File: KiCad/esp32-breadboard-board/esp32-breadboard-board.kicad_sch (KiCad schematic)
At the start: 23 parts, among them J1 USB_C_Receptacle_USB2.0_14P, J2 Conn_01x22_Pin, J3 Conn_01x22_Pin, SW1 BOOT, SW2 EN, U1 ESP32-S3-WROOM-1, U2 USBLC6-2SC6, U3 SGM2212-3.3XKC3G

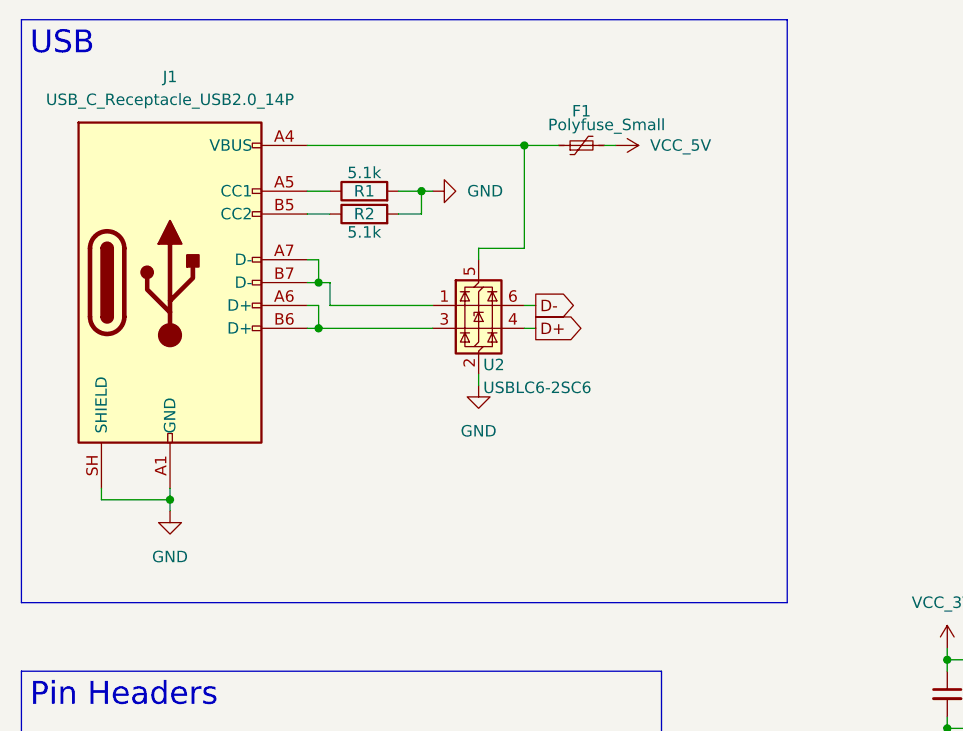
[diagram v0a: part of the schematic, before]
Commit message: Journal P2
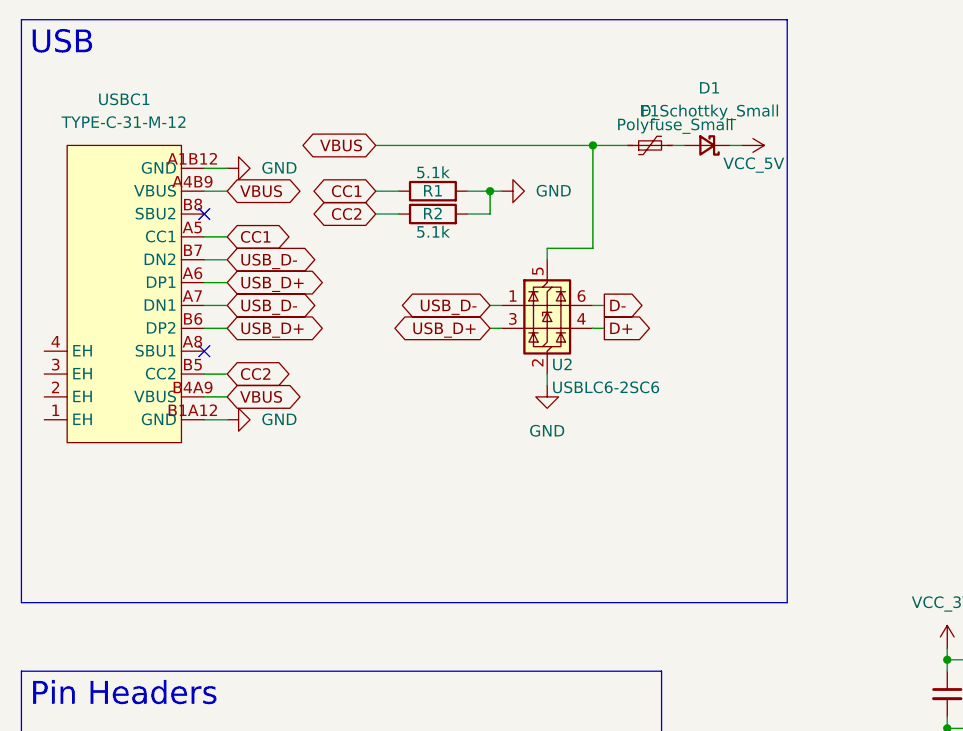
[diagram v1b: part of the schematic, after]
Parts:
- removed J1: USB_C_Receptacle_USB2.0_14P, symbol Connector:USB_C_Receptacle_USB2.0_14P
- added D1: D_Schottky_Small, easyeda2kicad:SOD-123_L2.7-W1.6-LS3.7-RD, symbol Device:D_Schottky_Small
- added USBC1: TYPE-C-31-M-12, easyeda2kicad:USB-C_SMD-TYPE-C-31-M-12_1, symbol easyeda2kicad:TYPE-C-31-M-12
- C10, C11, C7: footprint (none) -> Capacitor_SMD:C_0603_1608Metric
- C12, C14, C8, C9: footprint (none) -> Capacitor_SMD:C_0402_1005Metric
- D5: footprint (none) -> LED_SMD:LED_0603_1608Metric
- F1: footprint (none) -> Fuse:Fuse_0402_1005Metric
- J2, J3: footprint (none) -> Connector_PinHeader_2.54mm:PinHeader_1x20_P2.54mm_Vertical
- R1, R2, R3, R4, R5, R6: footprint (none) -> Resistor_SMD:R_0402_1005Metric
- SW1, SW2: footprint (none) -> easyeda2kicad:SW-SMD_L3.9-W3.0-P4.45
- U1: footprint RF_Module:ESP32-S3-WROOM-1 -> easyeda2kicad:WIFIM-SMD_ESP32-S3-WROOM-1-N8
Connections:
- net GND: now also USBC1.A1B12 (GND), USBC1.B1A12 (GND)
- net VCC_5V: now also D1.1 (K); no longer F1.2
- net VBUS: now reaches F1.1, U2.5 (VBUS)
- net VBUS: now also USBC1.A4B9 (VBUS), USBC1.B4A9 (VBUS)
- net CC1: now reaches R1.1
- net CC1: now also USBC1.A5 (CC1)
- net USB_D+: now reaches U2.3 (I/O2)
- net USB_D+: now also USBC1.A6 (DP1), USBC1.B6 (DP2)
- net USB_D-: now reaches U2.1 (I/O1)
- net USB_D-: now also USBC1.A7 (DN1), USBC1.B7 (DN2)
- net CC2: now reaches R2.1
- net CC2: now also USBC1.B5 (CC2)
- new net: D1.2 (A), F1.2
- no-connect marks 0 -> 2
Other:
- moved on the sheet: F1, R1, R2, U2
